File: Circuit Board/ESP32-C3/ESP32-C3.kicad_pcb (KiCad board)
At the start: 2 copper layers, 48 parts, among them IC1 W25Q16JVUXIQ_TR, J1 Conn_01x04_Male, J2 USB_C_Receptacle_USB2.0, SW1 SW_Push, SW2 SW_Push, U1 USBLC6-2SC6, U2 ESP32-C3, U3 USBLC6-2SC6, U4 SPX3819M5-L-3-3

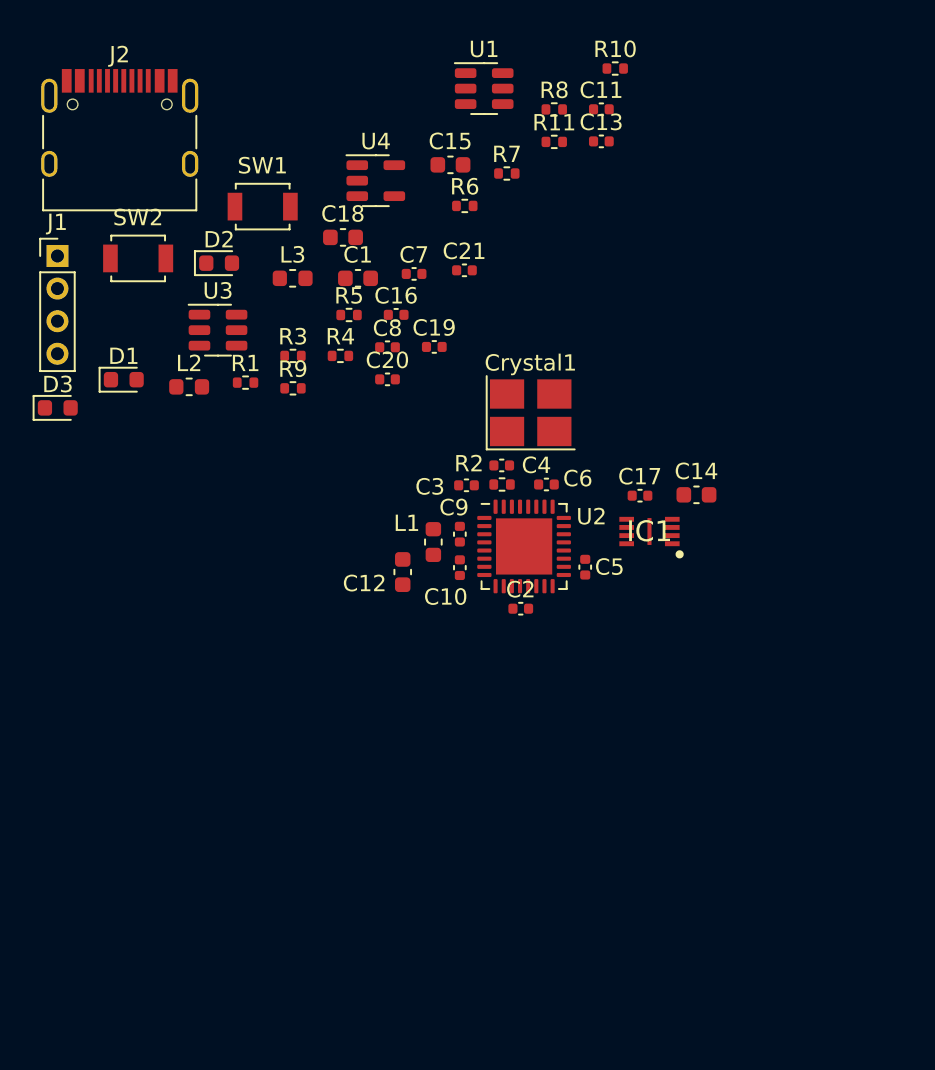
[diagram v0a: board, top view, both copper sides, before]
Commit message: Finished PCB Layout v1.0
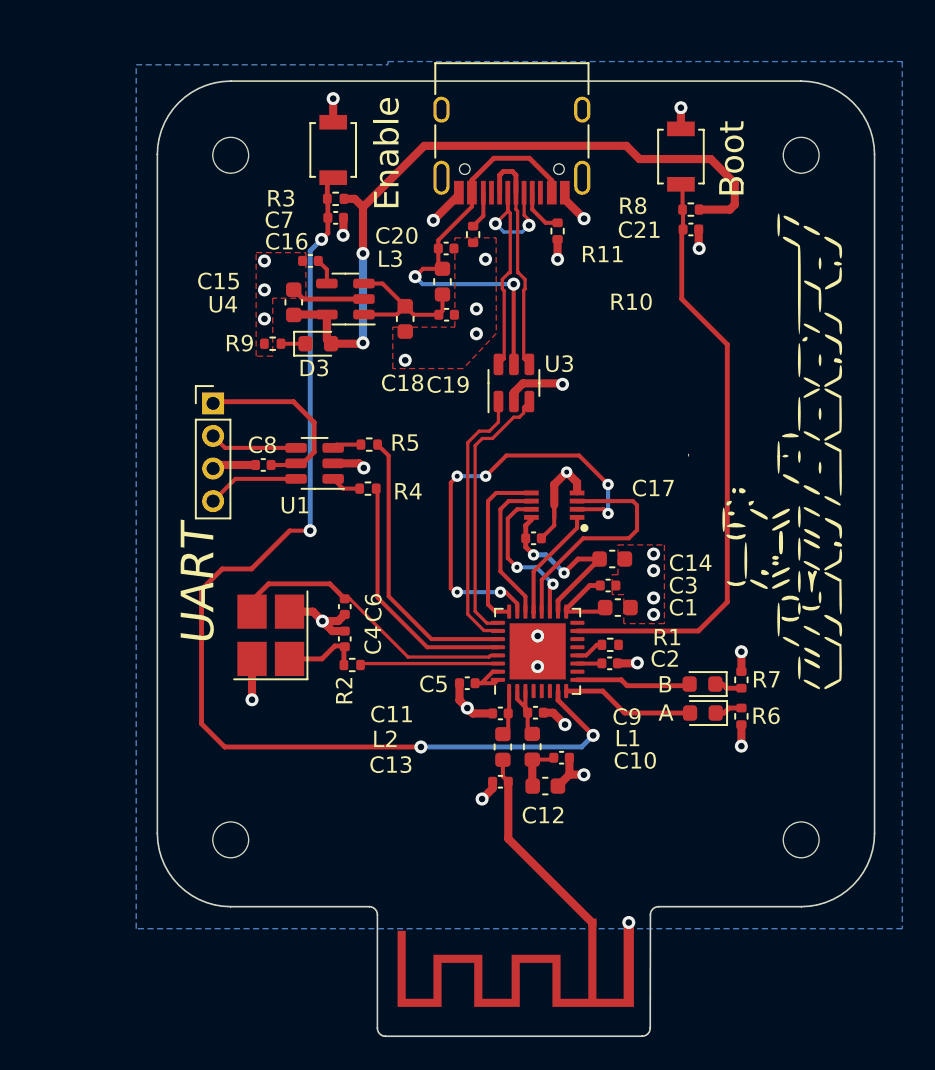
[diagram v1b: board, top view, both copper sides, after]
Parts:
- added ANT1: ESP32_Antenna, ESP32 Ant:ESPRESSIF_ESP32_MIFA_2.4GHz_Right, F.Cu at (72.0, 87.1)
- added G***: LOGO, LOGO, F.Cu at (82.4, 63.6)
- added G***: LOGO, LOGO, F.Cu at (85.4, 57.6)
- added G***: LOGO, LOGO, B.Cu at (83.4, 64.8)
- added G***: LOGO, LOGO, B.Cu at (86.4, 70.8)
- added H1: MountingHole, MountingHole:MountingHole_2.2mm_M2, F.Cu at (85.0, 40.0)
- added H2: MountingHole, MountingHole:MountingHole_2.2mm_M2, F.Cu at (50.0, 40.0)
- added H3: MountingHole, MountingHole:MountingHole_2.2mm_M2, F.Cu at (50.0, 82.0)
- added H4: MountingHole, MountingHole:MountingHole_2.2mm_M2, F.Cu at (85.0, 82.0)
- moved A 41.0 mm to (79.0, 74.2), turned to 180 degrees
- moved C13 39.8 mm to (66.5, 78.4), turned to 180 degrees
- moved B 39.3 mm to (78.9, 72.4), turned to 180 degrees
- moved C11 37.6 mm to (66.5, 74.2), turned to 180 degrees
- moved R6 35.6 mm to (81.3, 74.4), turned to -90 degrees
- moved R7 34.2 mm to (81.3, 72.2), turned to 90 degrees
- moved SW2 33.9 mm to (77.6, 40.1), turned to 90 degrees
- moved L2 29.3 mm to (66.7, 76.3), turned to -90 degrees
- moved R1 27.6 mm to (73.3, 70.0), turned to 180 degrees
- moved C1 25.7 mm to (73.8, 67.8)
- moved U1 25.2 mm to (55.1, 58.9), turned to 180 degrees
- moved J2 24.1 mm to (67.2, 38.2), turned to 180 degrees
- moved Crystal1 21.0 mm to (52.5, 69.5), turned to 90 degrees
- moved U3 18.4 mm to (67.4, 54.0), turned to 90 degrees
- moved D3 16.5 mm to (55.4, 51.6)
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- renumbered D1 to A, D2 to B
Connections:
- net Net-(C14-Pad2) renamed /VDD_SPI
- net Net-(C21-Pad1) renamed /BOOT
- net Net-(J2-PadA5) renamed /CC1
- net Net-(J2-PadA6) renamed /D+
- net Net-(J2-PadA7) renamed /D-
- net Net-(J2-PadB5) renamed /CC2
- C18 pad 1: GND -> /VBUS FILT
- C19 pad 1: GND -> /VBUS FILT
- C19 pad 2: Net-(C19-Pad2) -> GND
- C20 pad 1: GND -> /VBUS
- C20 pad 2: Net-(C20-Pad2) -> GND
- J2 pad A4: Net-(C20-Pad2) -> /VBUS
- J2 pad A9: Net-(C20-Pad2) -> /VBUS
- J2 pad B4: Net-(C20-Pad2) -> /VBUS
- J2 pad B9: Net-(C20-Pad2) -> /VBUS
- L3 pad 1: Net-(C19-Pad2) -> /VBUS FILT
- L3 pad 2: Net-(C20-Pad2) -> /VBUS
- U3 pad 5: Net-(C20-Pad2) -> /VBUS
- U4 pad 1: GND -> /VBUS FILT
- U4 pad 3: GND -> /VBUS FILT
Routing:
- net /CHIP_EN: track 0.00 -> 67.2 mm, vias 0 -> 4
- net GND: track 0.00 -> 52.7 mm, vias 0 -> 33
- net +3.3V: track 0.00 -> 47.3 mm, vias 0 -> 2
- net /BOOT: track 0.00 -> 36.8 mm
- net SPI_DI: track 0.00 -> 26.3 mm, vias 0 -> 6
- net /VBUS: track 0.00 -> 26.2 mm, vias 0 -> 2
- net /UART0_RX: track 0.00 -> 19.2 mm
- net /XTAL_N: track 0.00 -> 18.1 mm
- net /D-: track 0.00 -> 17.8 mm, vias 0 -> 2
- net /UART0_TX: track 0.00 -> 17.2 mm
- net /USB_D-: track 0.00 -> 16.5 mm
- net /USB_D+: track 0.00 -> 16.5 mm
- net SPI_NWP: track 0.00 -> 14.4 mm
- net /D+: track 0.00 -> 14.3 mm
- net +3.3VA: track 0.00 -> 13.6 mm
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- added copper zone on B.Cu, net GND
- added copper zone on F.Cu, net GND
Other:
- board outline added: 44 x 58.6 mm
- board text added: "Boot"
- board text added: "Enable"
- board text added: "UART"
- board text added: "V1.0 May 2023"
